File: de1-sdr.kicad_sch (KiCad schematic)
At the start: 181 parts, among them J1 RF IN, J2 DE1-HEADER, J3 UFL, Q1 BSS138, Q2 AO3401A, T1 TC4-1TX+, U1 AD9609-80, U10 TPS7A2018DBV, U11 TPS7A2033DBV, U12 TPS7A2033DBV, U13 TPS7A2033DBV, U2 QPL9547, U3 MAX2682, U4 LMX2594, U5 BDA4620, U6 TPS7A2018DBV, U7 PAT1220-C-2DB, U8 BG18C, U9 BG18C, Y1 ECS-3518-800-B-TR

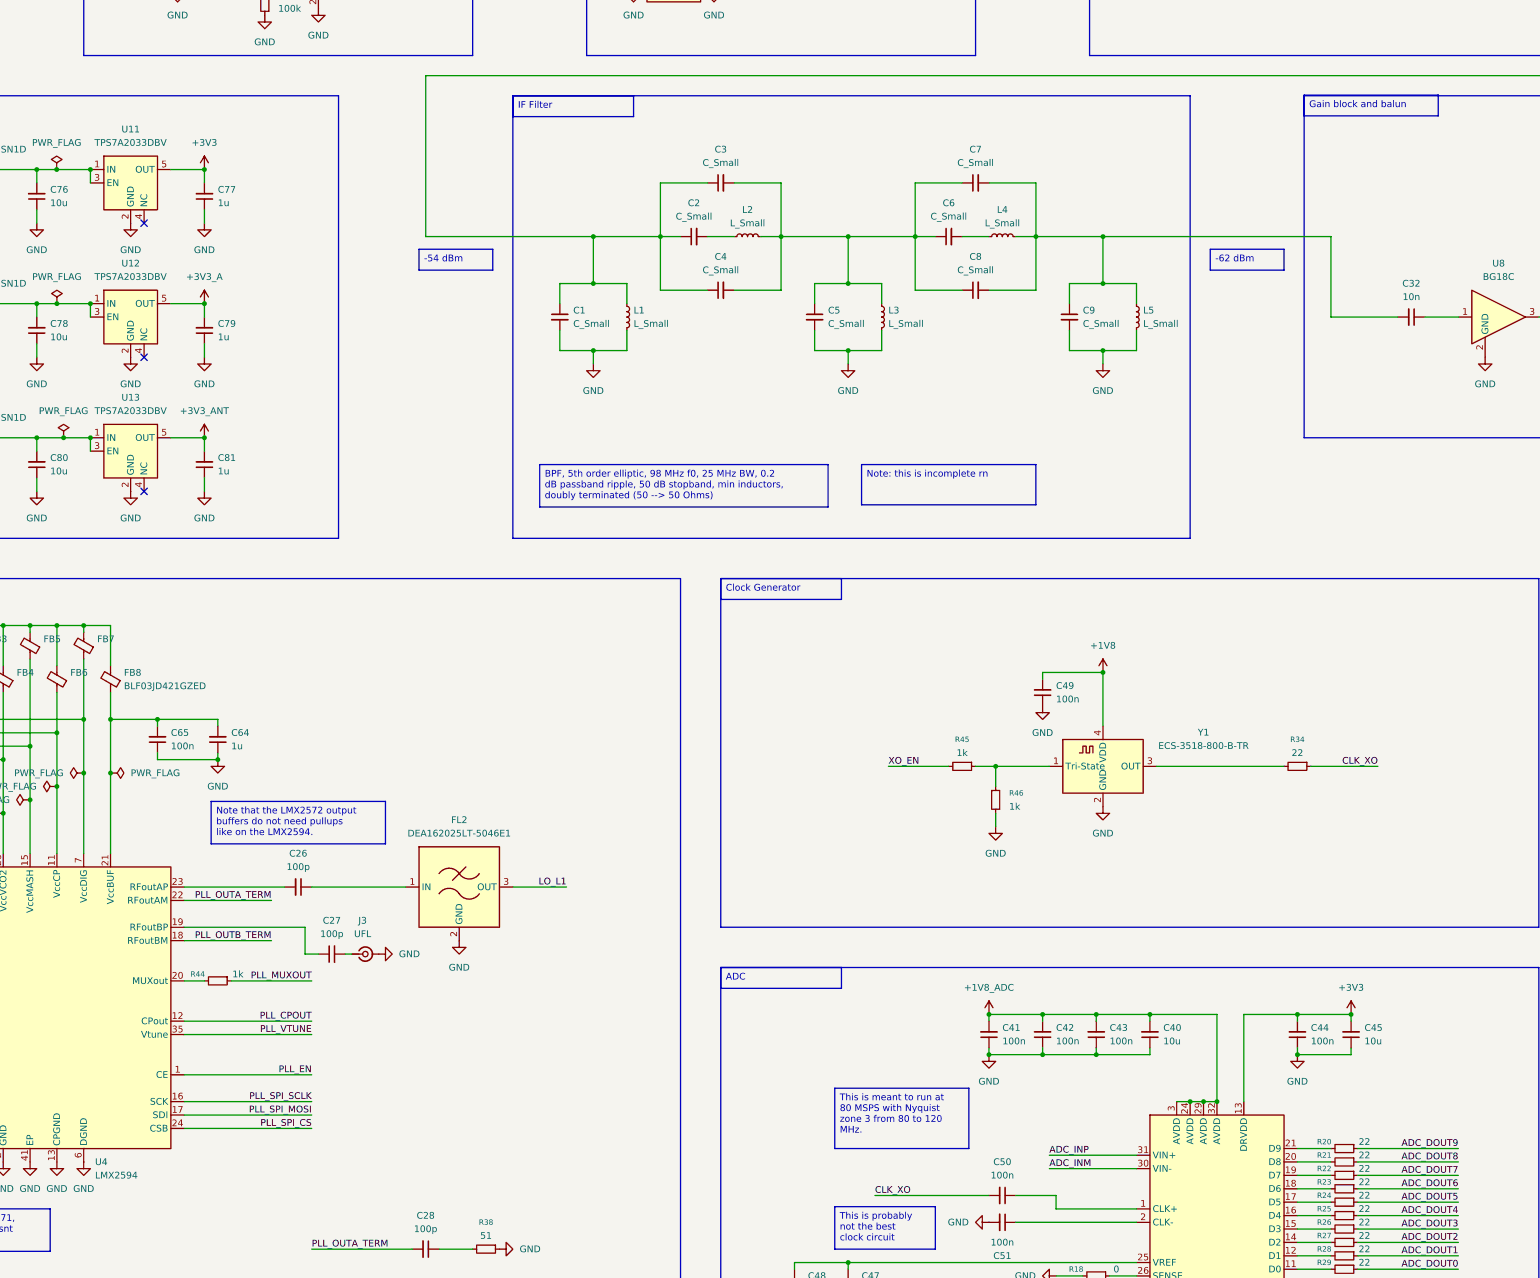
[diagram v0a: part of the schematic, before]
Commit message: fix more typo
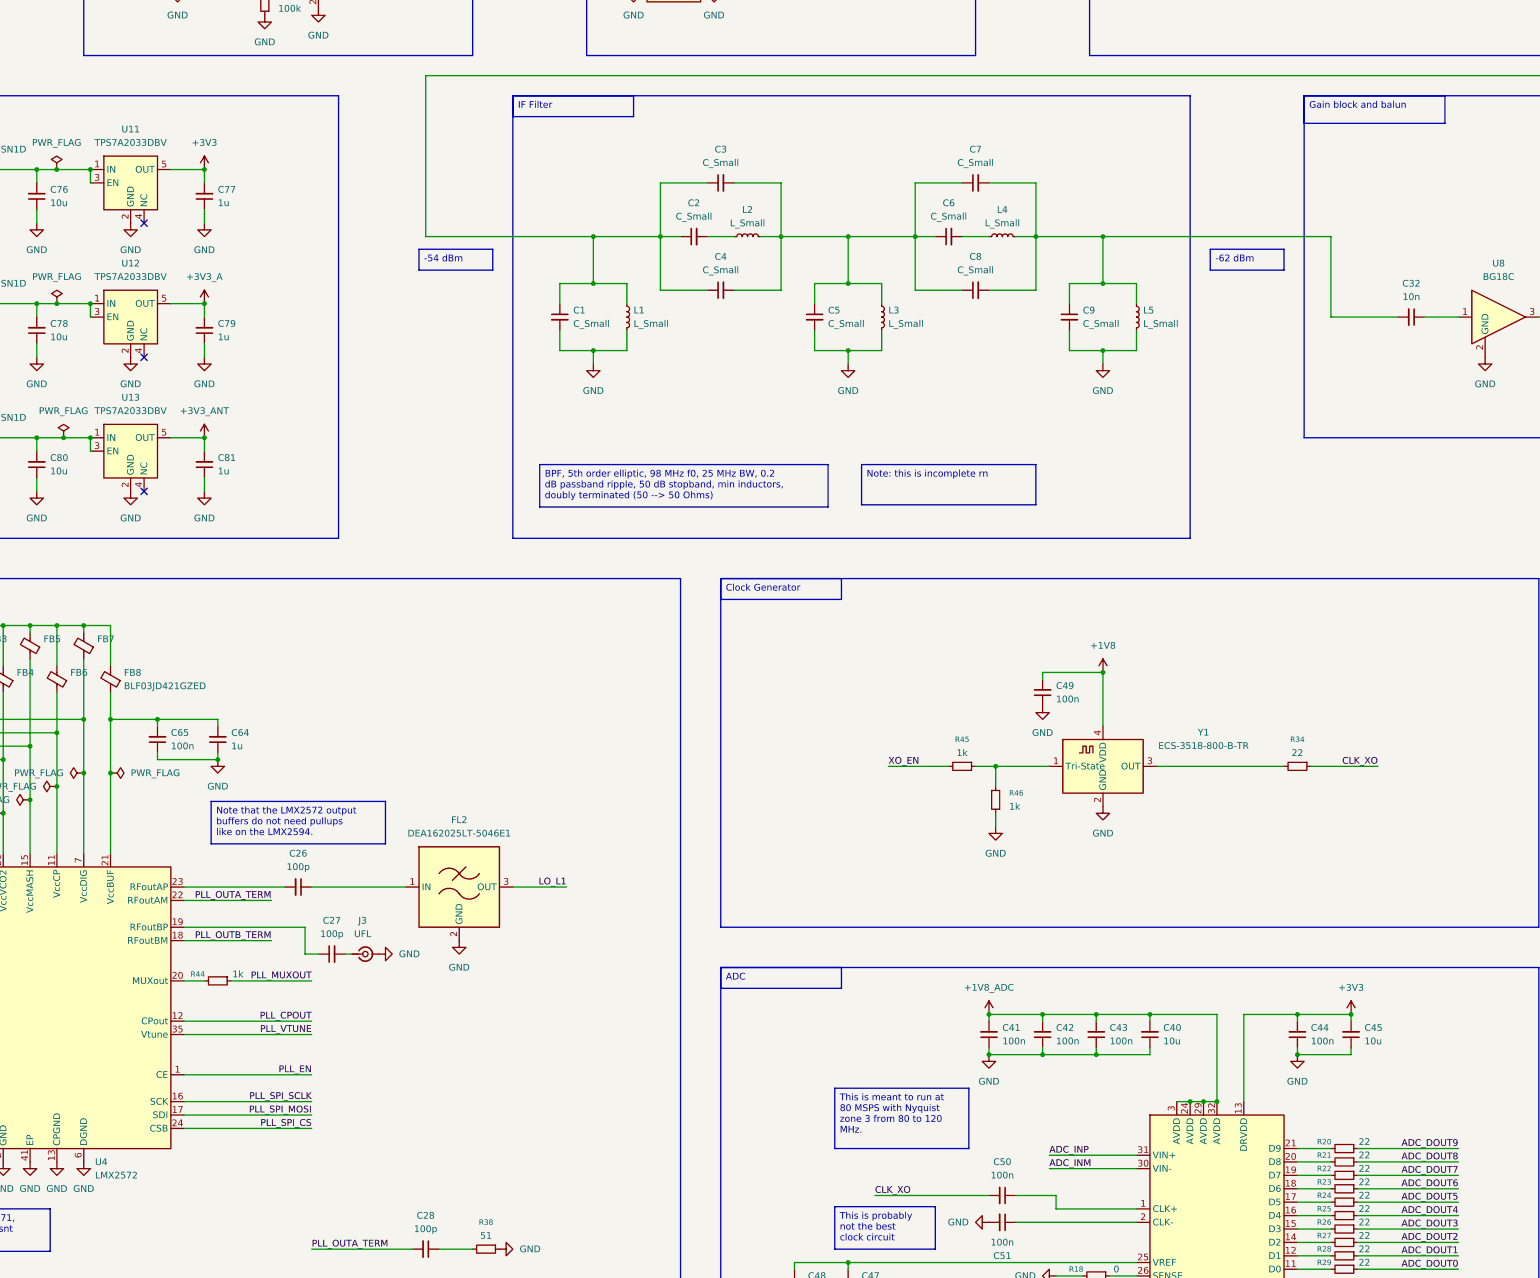
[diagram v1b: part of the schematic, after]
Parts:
- U4: value LMX2594 -> LMX2572
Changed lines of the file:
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@@
 	(text_box "Gain block and balun"
 		(exclude_from_sim no)
-		(at 393.7 129.4017 0)
-		(size 25.4 3.9483)
+		(at 393.7 129.54 0)
+		(size 26.67 5.2183)
 		(margins 0.9525 0.9525 0.9525 0.9525)
 		(stroke
@@
 			)
 		)
-		(property "Value" "LMX2594"
+		(property "Value" "LMX2572"
 			(at 164.7033 334.01 0)
 			(show_name no)
@@
 			)
 		)
-		(property "Datasheet" "https://www.ti.com/lit/ds/symlink/lmx2594.pdf"
+		(property "Datasheet" ""
 			(at 154.94 302.26 0)
 			(hide yes)
@@
 			)
 		)
-		(property "Description" "LMX2594 15-GHz Wideband PLLATINUM™ RF Synthesizer With Phase Synchronization and JESD204B Support"
+		(property "Description" ""
 			(at 154.94 302.26 0)
 			(hide yes)

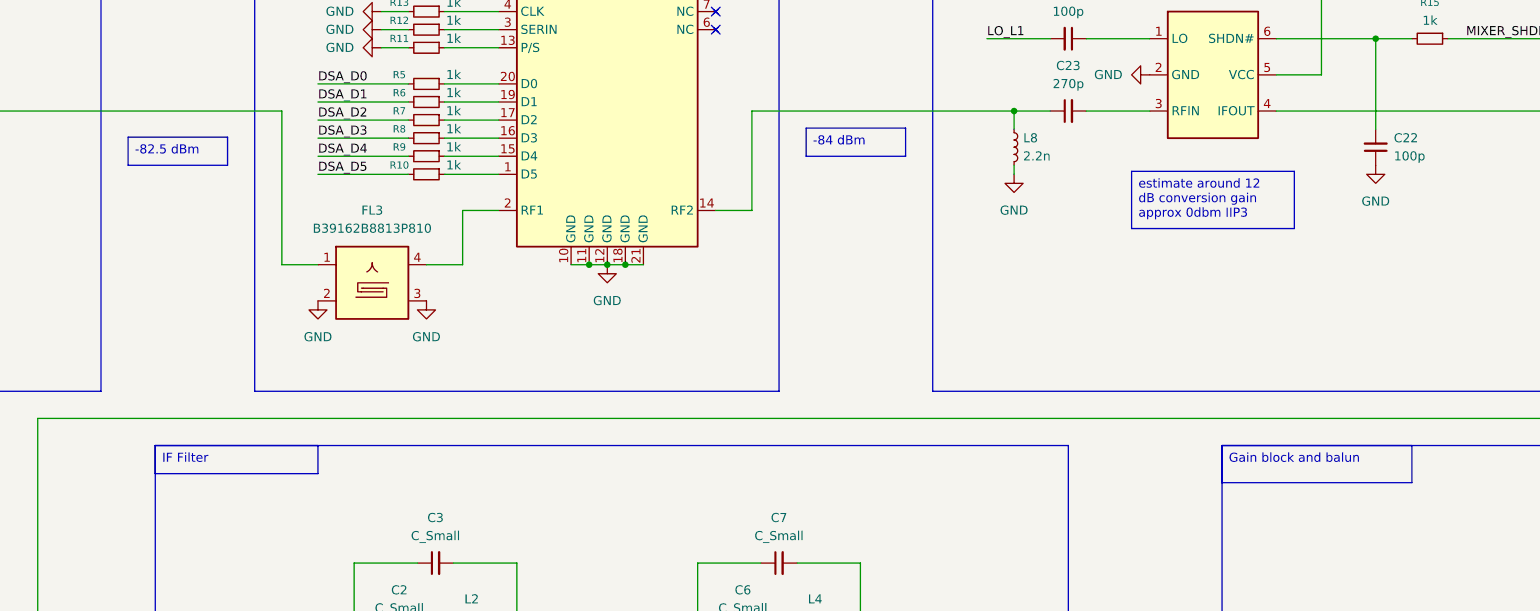
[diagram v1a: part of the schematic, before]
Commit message: fix more typo
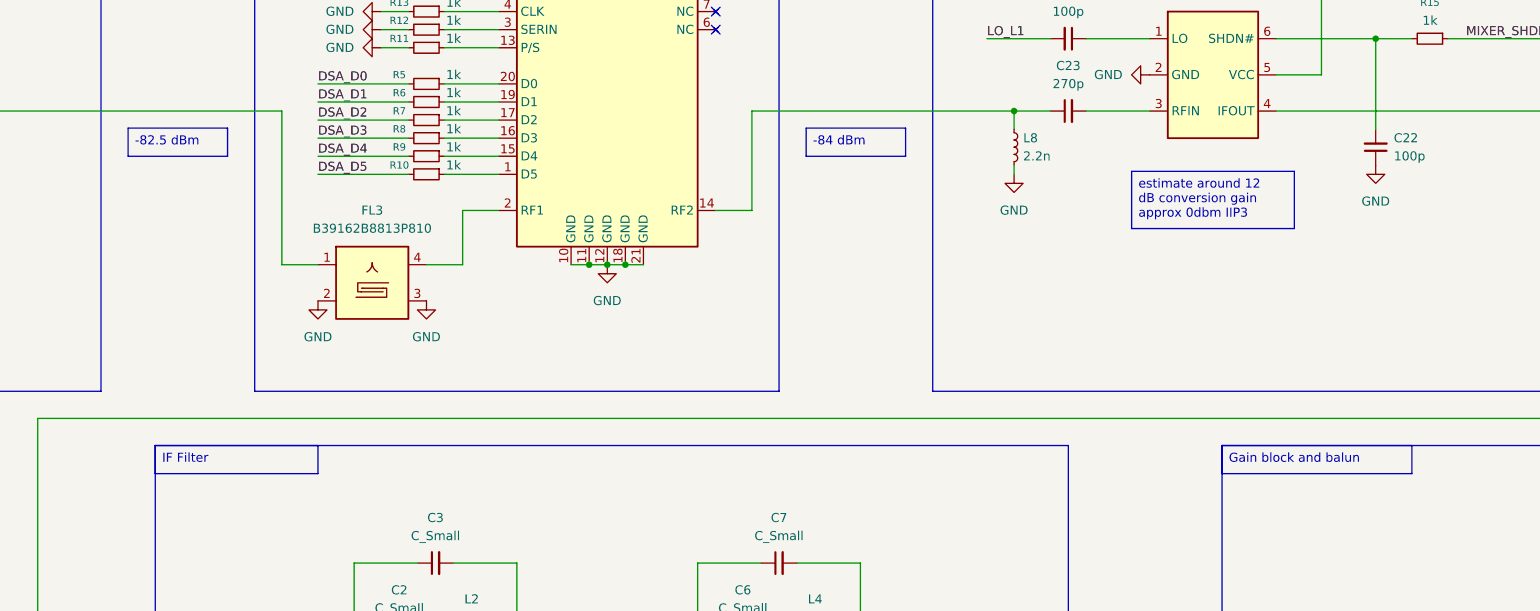
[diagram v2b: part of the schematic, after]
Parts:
- U4: footprint Package_DFN_QFN:VQFN-40-1EP_6x6mm_P0.5mm_EP3.5x3.5mm_ThermalVias -> Package_DFN_QFN:HVQFN-40-1EP_6x6mm_P0.5mm_EP4.1x4.1mm
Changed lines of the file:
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@@
 		(exclude_from_sim no)
 		(at 393.7 129.54 0)
-		(size 26.67 5.2183)
+		(size 26.67 3.9483)
 		(margins 0.9525 0.9525 0.9525 0.9525)
 		(stroke
@@
 	(text_box "-82.5 dBm"
 		(exclude_from_sim no)
-		(at 240.03 86.2217 0)
+		(at 240.03 84.9517 0)
 		(size 13.97 3.9483)
 		(margins 0.9525 0.9525 0.9525 0.9525)
@@
 			)
 		)
-		(property "Footprint" "Package_DFN_QFN:VQFN-40-1EP_6x6mm_P0.5mm_EP3.5x3.5mm_ThermalVias"
+		(property "Footprint" "Package_DFN_QFN:HVQFN-40-1EP_6x6mm_P0.5mm_EP4.1x4.1mm"
 			(at 154.94 302.26 0)
 			(hide yes)
@@
 			)
 		)
-		(property "Datasheet" ""
+		(property "Datasheet" "https://www.ti.com/lit/ds/symlink/lmx2572.pdf"
 			(at 154.94 302.26 0)
 			(hide yes)
@@
 			)
 		)
-		(property "Description" ""
+		(property "Description" "LMX2572 6.4-GHz Low power wideband RF synthesizer with phase synchronization and JESD204B support"
 			(at 154.94 302.26 0)
 			(hide yes)
